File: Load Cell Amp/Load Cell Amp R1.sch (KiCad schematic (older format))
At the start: 37 parts, among them J1 Conn_01x02_Male, J2 Conn_01x02_Male, J3 Conn_01x02_Male, J4 Conn_01x02_Male, J5 Conn_01x02_Male, J6 Conn_02x06_Odd_Even, J7 DB-26, U1 AD8227, U10 OP1177, U11 OP1177, U12 OP1177, U2 AD8227, U3 AD8227, U4 AD8227, U5 AD8227, U6 AD8227, U7 OP1177, U8 OP1177, U9 OP1177

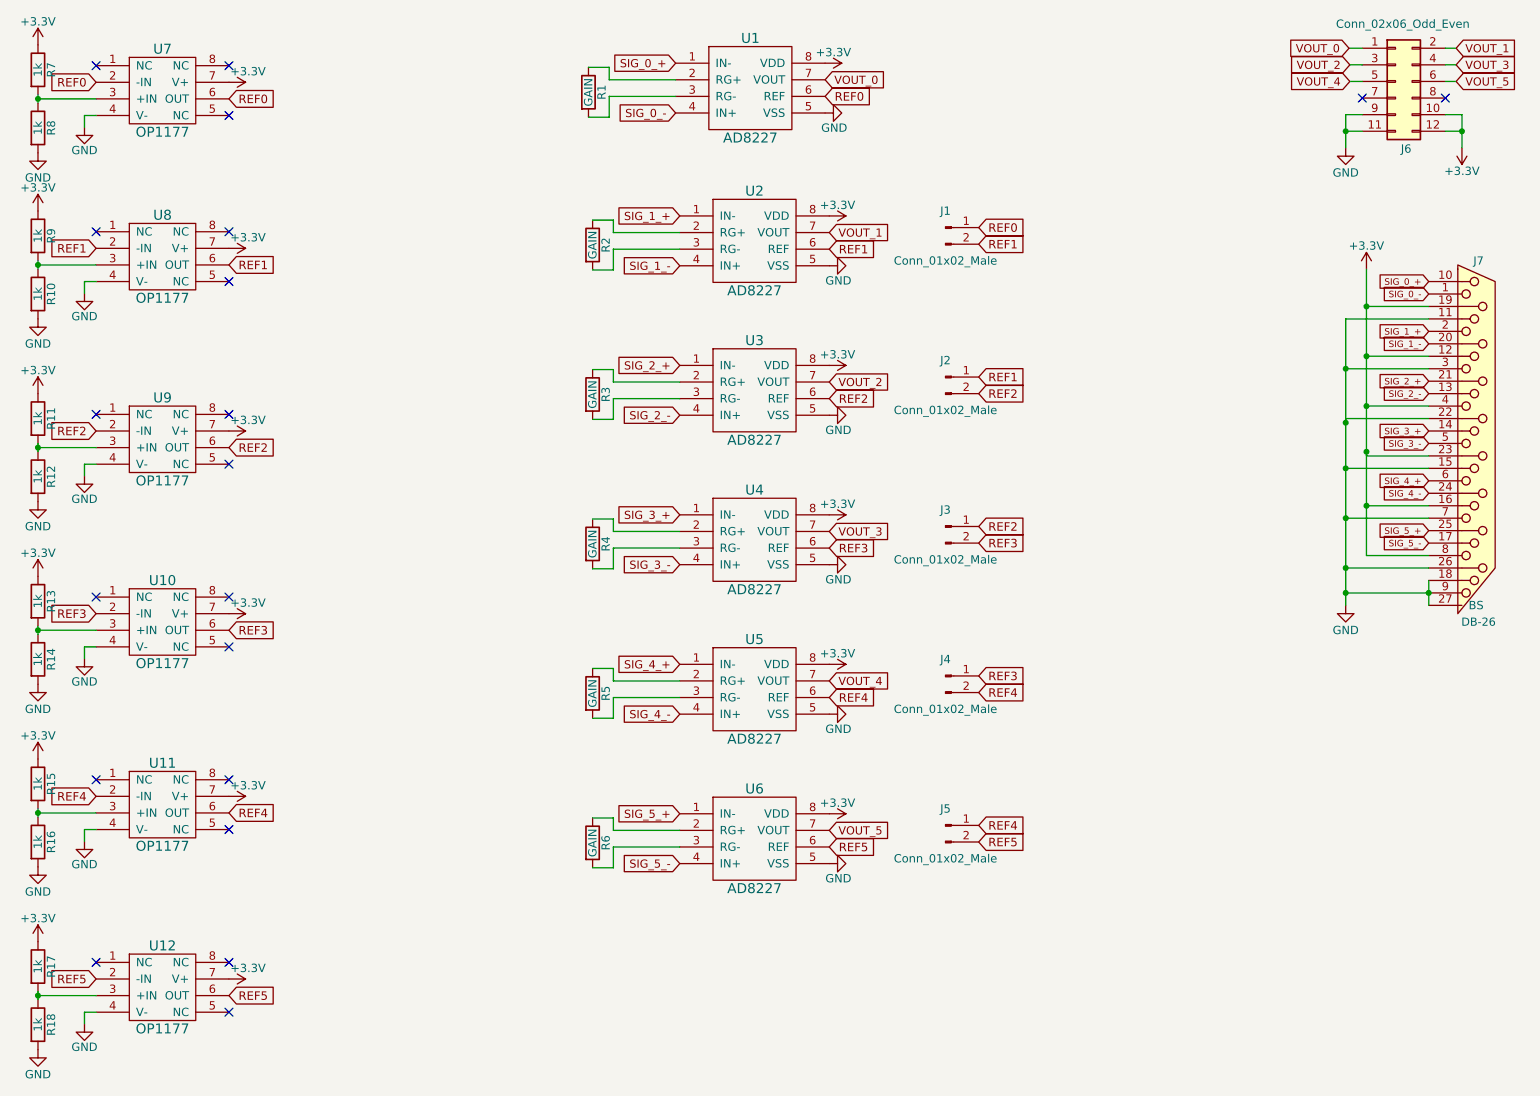
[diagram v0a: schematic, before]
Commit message: edits1
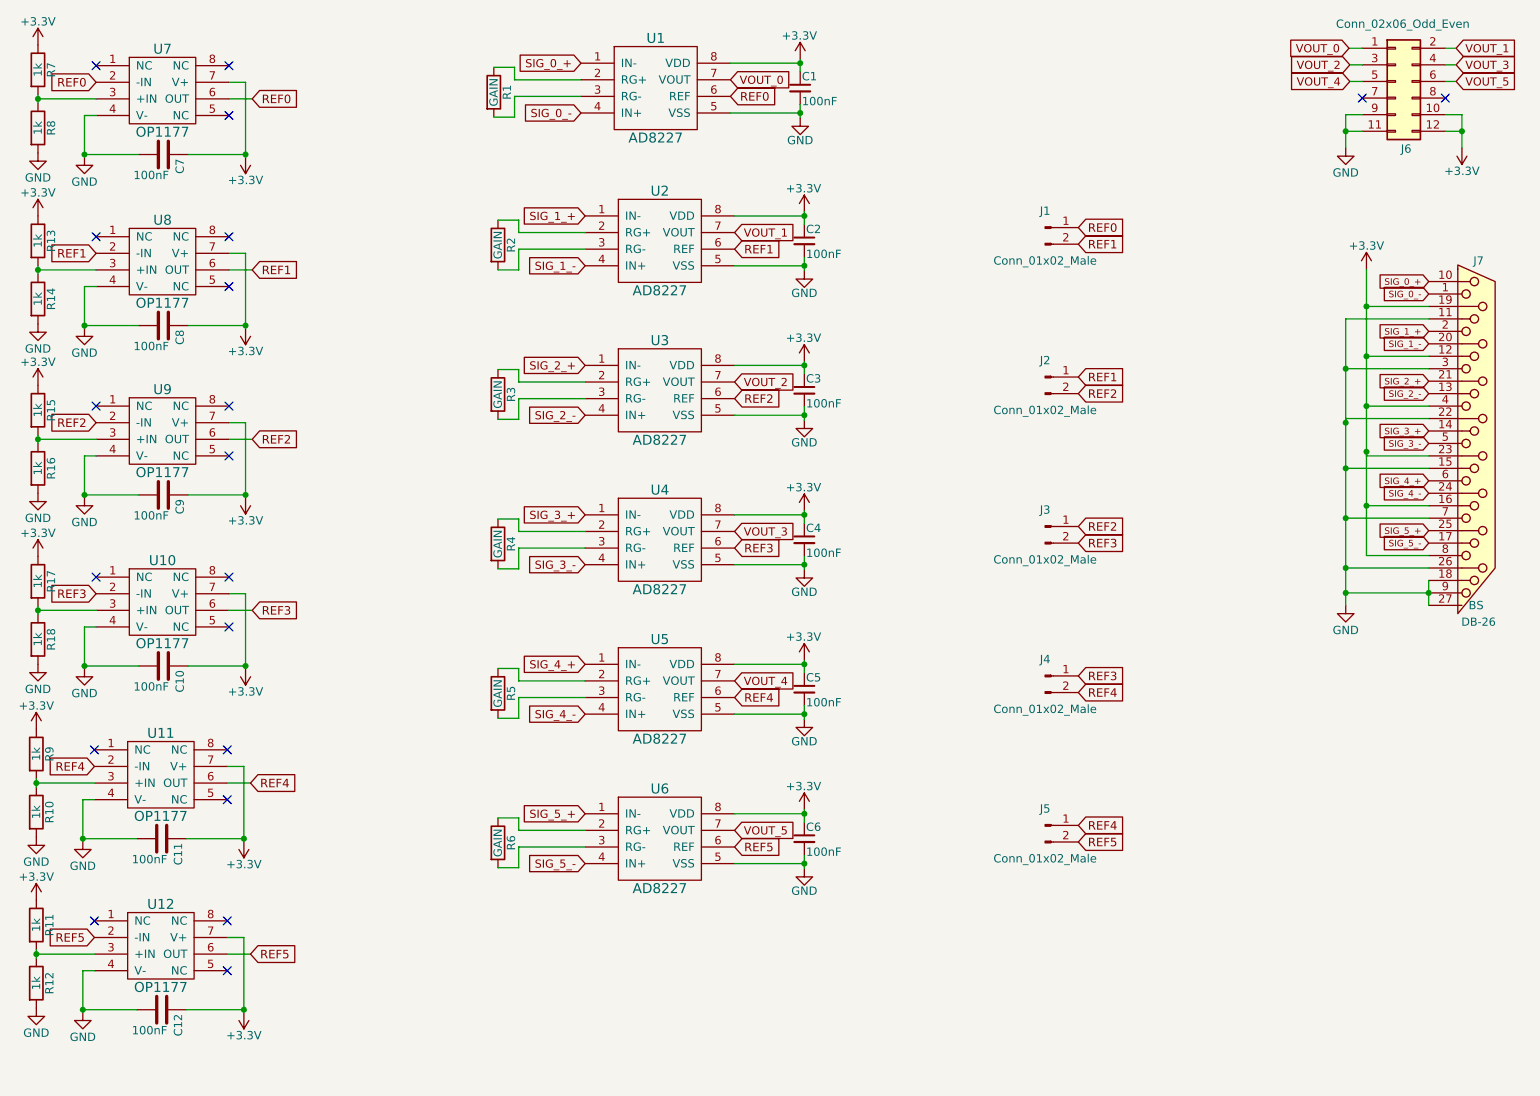
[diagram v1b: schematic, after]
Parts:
- added C1, C2, C3, C4, C5, C6: 100nF, Capacitors_SMD:C_0805, symbol C_Small
- added C10, C11, C12, C7, C8, C9: 100nF, Capacitors_SMD:C_0805, symbol C
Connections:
- net +3V3: now also C1.1, C10.1, C11.1, C12.1, C2.1, C3.1, C4.1, C5.1, C6.1, C7.1, C8.1, C9.1
- net GND: now also C1.2, C10.2, C11.2, C12.2, C2.2, C3.2, C4.2, C5.2, C6.2, C7.2, C8.2, C9.2
- net at R10.1, R9.2: now also U11.3 (+IN); no longer U8.3 (+IN)
- net at R11.2, R12.1: now also U12.3 (+IN); no longer U9.3 (+IN)
- net at R13.2, R14.1: now also U8.3 (+IN); no longer U10.3 (+IN)
- net at R15.2, R16.1: now also U9.3 (+IN); no longer U11.3 (+IN)
- net at R17.2, R18.1: now also U10.3 (+IN); no longer U12.3 (+IN)
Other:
- moved on the sheet: J1, J2, J3, J4, J5, R1, R2, R3, R4, R5, R6, U1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
